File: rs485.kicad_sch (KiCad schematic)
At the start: 9 parts, among them U7 ISL3172EIUZ

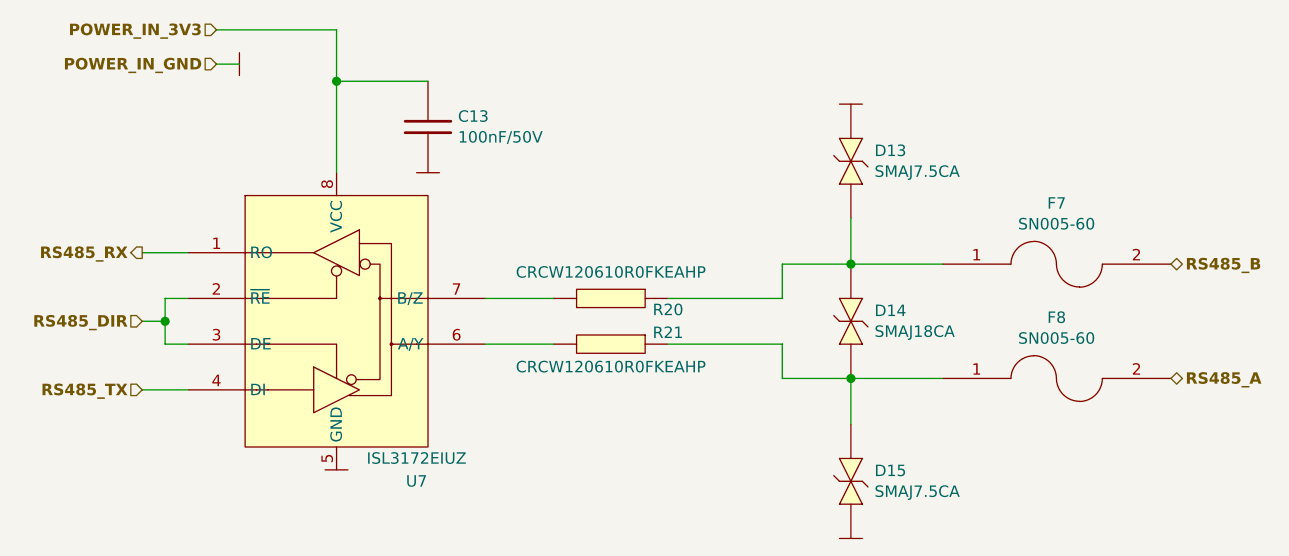
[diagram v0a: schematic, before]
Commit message: Finalized project
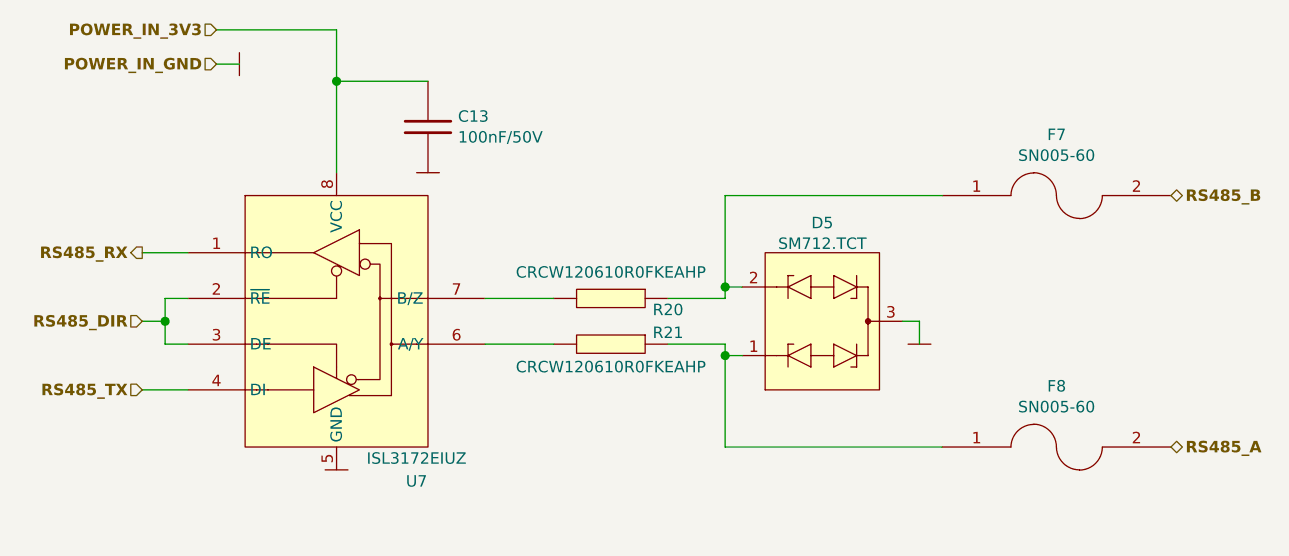
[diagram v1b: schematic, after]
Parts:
- removed D13, D15: SMAJ7.5CA, Diodes:SMAJ7.5CA_SMD_DO214AC, symbol Diodes:SMAJ7.5CA
- removed D14: SMAJ18CA, Diodes:SMAJ18CA_SMD_DO214AC, symbol Diodes:SMAJ18CA
- added D5: SM712.TCT, ESD_Protectors:SM712.TCT, symbol esd_protectors:SM712.TCT
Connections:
- net GND: now also D5.3 (GND)
- net at F8.1, R21.1: now also D5.1 (I/O1)
- net at F7.1, R20.1: now also D5.2 (I/O2)
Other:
- moved on the sheet: F7, F8
